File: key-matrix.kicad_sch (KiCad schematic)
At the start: 168 parts, among them SW1 SW_Push_45deg, SW10 SW_Push_45deg, SW11 SW_Push_45deg, SW12 SW_Push_45deg, SW13 SW_Push_45deg, SW14 SW_Push_45deg, SW15 SW_Push_45deg, SW16 SW_Push_45deg, SW17 SW_Push_45deg, SW18 SW_Push_45deg, SW19 SW_Push_45deg, SW2 SW_Push_45deg, SW20 SW_Push_45deg, SW21 SW_Push_45deg, SW22 SW_Push_45deg, SW23 SW_Push_45deg, SW24 SW_Push_45deg, SW25 SW_Push_45deg, SW26 SW_Push_45deg, SW27 SW_Push_45deg, SW28 SW_Push_45deg, SW29 SW_Push_45deg, SW3 SW_Push_45deg, SW30 SW_Push_45deg, SW31 SW_Push_45deg, SW32 SW_Push_45deg, SW33 SW_Push_45deg, SW34 SW_Push_45deg, SW35 SW_Push_45deg, SW36 SW_Push_45deg, SW37 SW_Push_45deg, SW38 SW_Push_45deg, SW39 SW_Push_45deg, SW4 SW_Push_45deg, SW40 SW_Push_45deg, SW41 SW_Push_45deg, SW42 SW_Push_45deg, SW43 SW_Push_45deg, SW44 SW_Push_45deg, SW45 SW_Push_45deg, SW46 SW_Push_45deg, SW47 SW_Push_45deg, SW48 SW_Push_45deg, SW49 SW_Push_45deg, SW5 SW_Push_45deg, SW50 SW_Push_45deg, SW51 SW_Push_45deg, SW52 SW_Push_45deg, SW53 SW_Push_45deg, SW54 SW_Push_45deg, SW55 SW_Push_45deg, SW56 SW_Push_45deg, SW57 SW_Push_45deg, SW58 SW_Push_45deg, SW59 SW_Push_45deg, SW6 SW_Push_45deg, SW60 SW_Push_45deg, SW61 SW_Push_45deg, SW62 SW_Push_45deg, SW63 SW_Push_45deg, SW64 SW_Push_45deg, SW65 SW_Push_45deg, SW66 SW_Push_45deg, SW67 SW_Push_45deg, SW68 SW_Push_45deg, SW69 SW_Push_45deg, SW7 SW_Push_45deg, SW70 SW_Push_45deg, SW71 SW_Push_45deg, SW72 SW_Push_45deg, SW73 SW_Push_45deg, SW74 SW_Push_45deg, SW75 SW_Push_45deg, SW76 SW_Push_45deg, SW77 SW_Push_45deg, SW78 SW_Push_45deg, SW79 SW_Push_45deg, SW8 SW_Push_45deg, SW80 SW_Push_45deg, SW81 SW_Push_45deg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

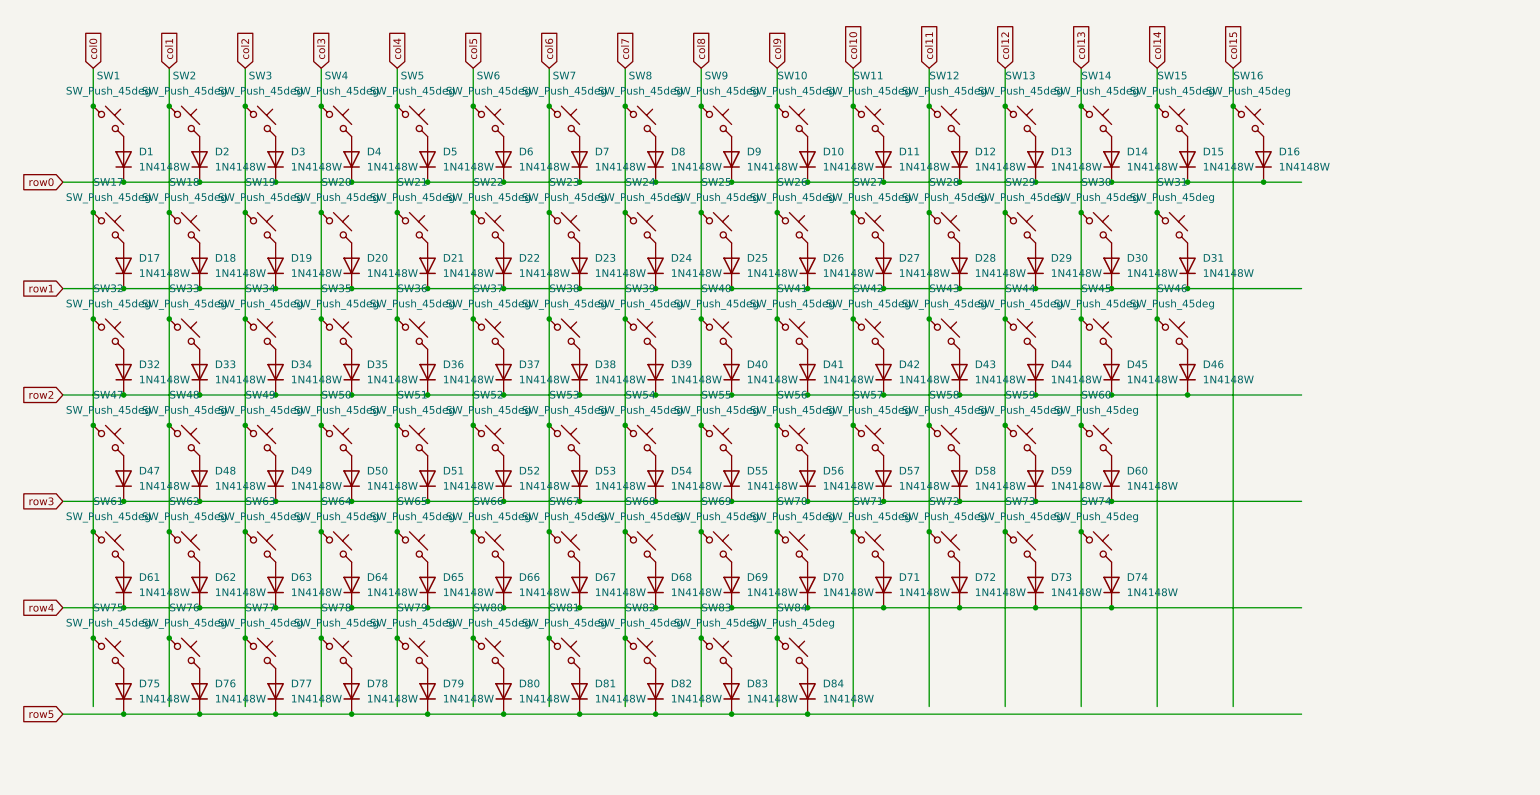
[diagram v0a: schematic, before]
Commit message: almost done
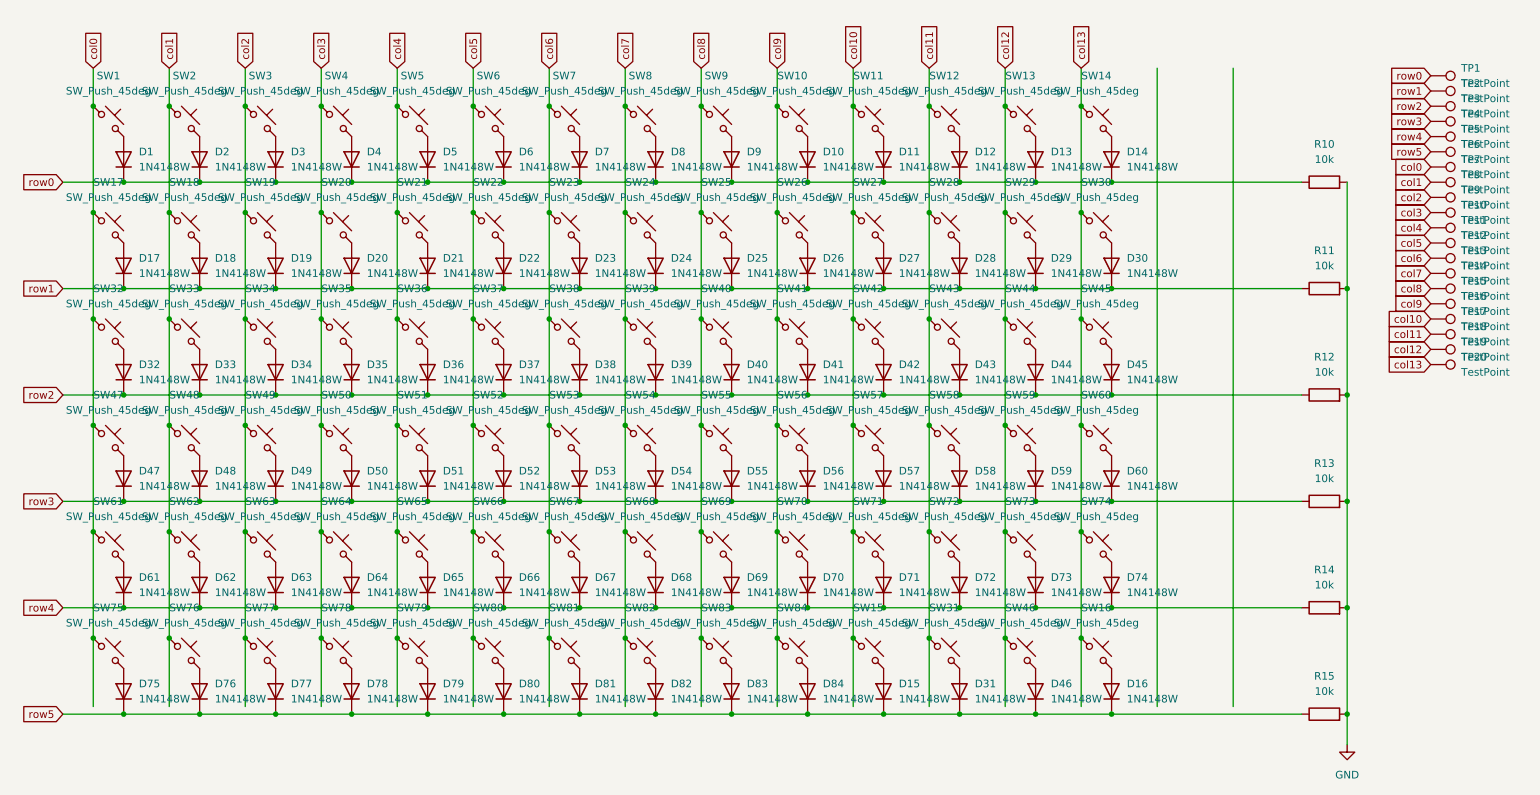
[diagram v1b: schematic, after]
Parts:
- added R10, R11, R12, R13, R14, R15: 10k, Resistor_SMD:R_0805_2012Metric_Pad1.20x1.40mm_HandSolder, symbol Device:R
- added TP1, TP10, TP11, TP12, TP13, TP14, TP15, TP16, TP17, TP18, TP19, TP2, TP20, TP3, TP4, TP5, TP6, TP7, TP8, TP9: TestPoint, TestPoint:TestPoint_Pad_D1.0mm, symbol Connector:TestPoint
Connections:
- net col15 is gone; now on net col13: SW16.1
- net col0: now also TP7.1
- net col1: now also TP8.1
- net col10: now also SW15.1, TP17.1
- net col11: now also SW31.1, TP18.1
- net col12: now also SW46.1, TP19.1
- net col13: now also TP20.1
- net col2: now also TP9.1
- net col3: now also TP10.1
- net col4: now also TP11.1
- net col5: now also TP12.1
- net col6: now also TP13.1
- net col7: now also TP14.1
- net col8: now also TP15.1
- net col9: now also TP16.1
- net row0: now also R10.1, TP1.1; no longer D15.1 (K), D16.1 (K)
- net row1: now also R11.1, TP2.1; no longer D31.1 (K)
- net row2: now also R12.1, TP3.1; no longer D46.1 (K)
- net row3: now also R13.1, TP4.1
- net row4: now also R14.1, TP5.1
- net row5: now also D15.1 (K), D16.1 (K), D31.1 (K), D46.1 (K), R15.1, TP6.1
- removed net col14: SW15.1, SW31.1, SW46.1
- new net GND: R10.2, R11.2, R12.2, R13.2, R14.2, R15.2
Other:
- moved on the sheet: D16, D31, D46, SW16, SW31, SW46
